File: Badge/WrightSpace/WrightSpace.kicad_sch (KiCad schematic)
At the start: 38 parts, among them J1 Conn_02x03_Counter_Clockwise, J3 Conn_02x03_Counter_Clockwise, J4 Conn_02x03_Counter_Clockwise, SW1 SW_SPDT, SW2 SW_SPDT, U1 ESP32-S2-SOLO

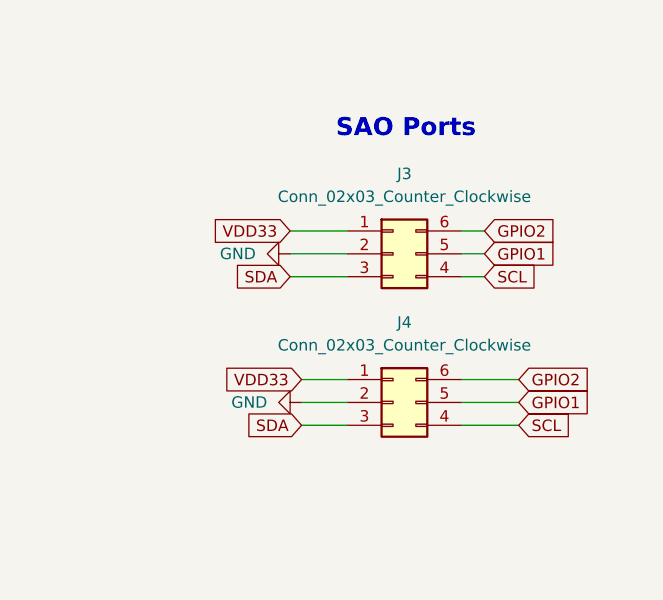
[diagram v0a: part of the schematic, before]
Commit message: refined artwork and poc WrightStuff
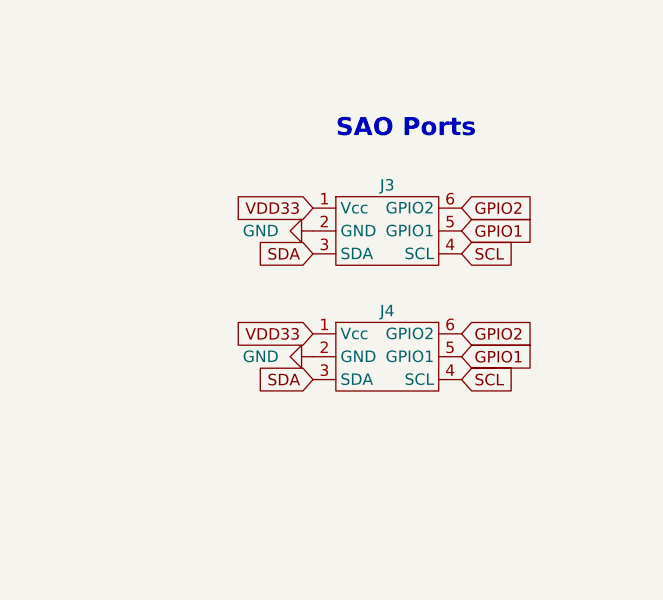
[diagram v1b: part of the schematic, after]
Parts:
- removed J3, J4: Conn_02x03_Counter_Clockwise, aerospace_badge:sao_1.69, symbol Connector_Generic:Conn_02x03_Counter_Clockwise
- added J3, J4: ~, aerospace_badge:sao_1.69, symbol av_Badge2023:SAO_v1.69
- J2: footprint Badge_Libraries:Wright X2 -> Badge_Libraries:Wright X3
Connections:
- net GND: now also J3.2 (GND), J4.2 (GND)
- net GPIO1: now also J3.5 (GPIO1), J4.5 (GPIO1)
- net GPIO2: now also J3.6 (GPIO2), J4.6 (GPIO2)
- net SCL: now also J3.4 (SCL), J4.4 (SCL)
- net SDA: now also J3.3 (SDA), J4.3 (SDA)
- net VDD33: now also J3.1 (Vcc), J4.1 (Vcc)

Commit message: artwork tweaks to get more into KiCad
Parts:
- D1, D2, D3, D4, D5, D6: footprint LED_SMD:LED_1206_3216Metric_ReverseMount_Hole1.8x2.4mm -> aerospace_badge:led_in-s124ar; MPN (none) -> IN-S124ARUW
- D7, D8: footprint LED_SMD:LED_Kingbright_APFA3010_3x1.5mm_Horizontal -> sunled:XZMDKCBDDG45S-9
